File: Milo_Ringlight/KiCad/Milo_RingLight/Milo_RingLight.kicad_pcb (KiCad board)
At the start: 2 copper layers, 16 parts, among them J1 Barrel_Jack_MountingPin, J2 MountingHole, J3 MountingHole, J4 MountingHole, J5 MountingHole, J6 Power Connector

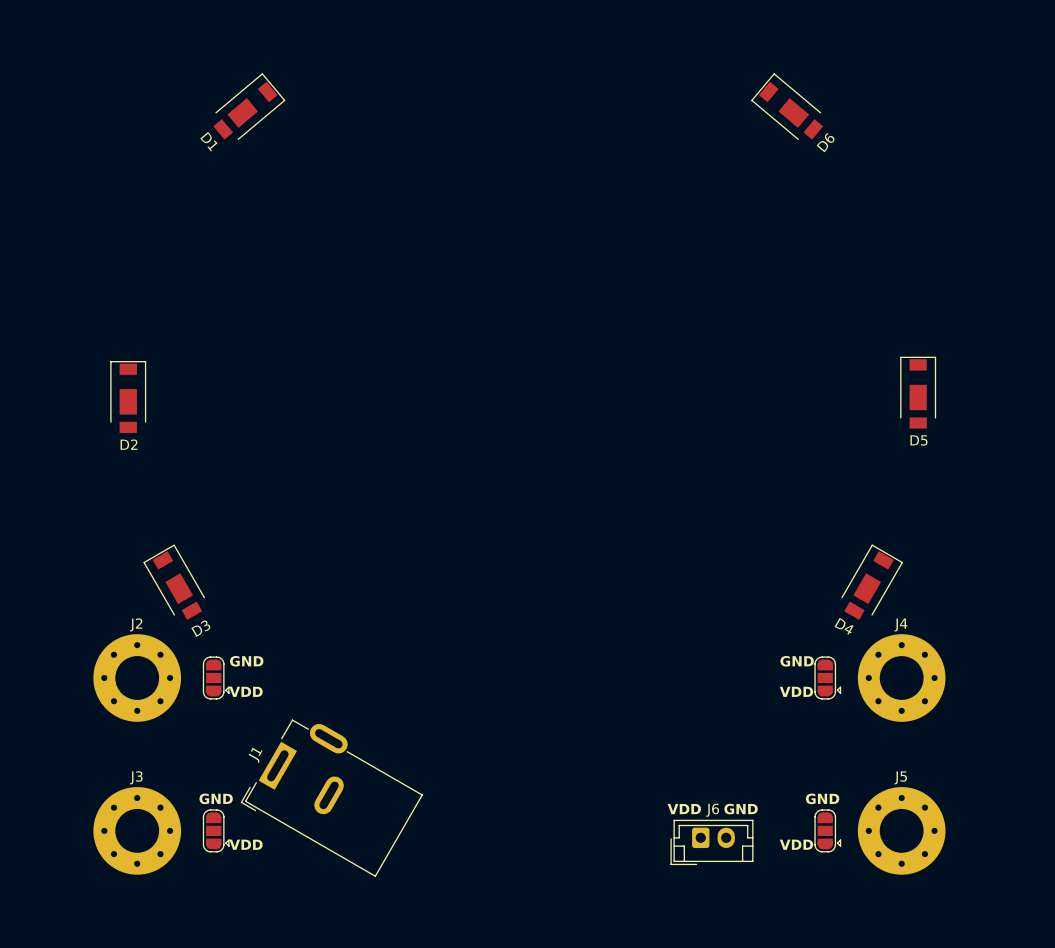
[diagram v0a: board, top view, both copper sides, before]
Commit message: Continued Work.
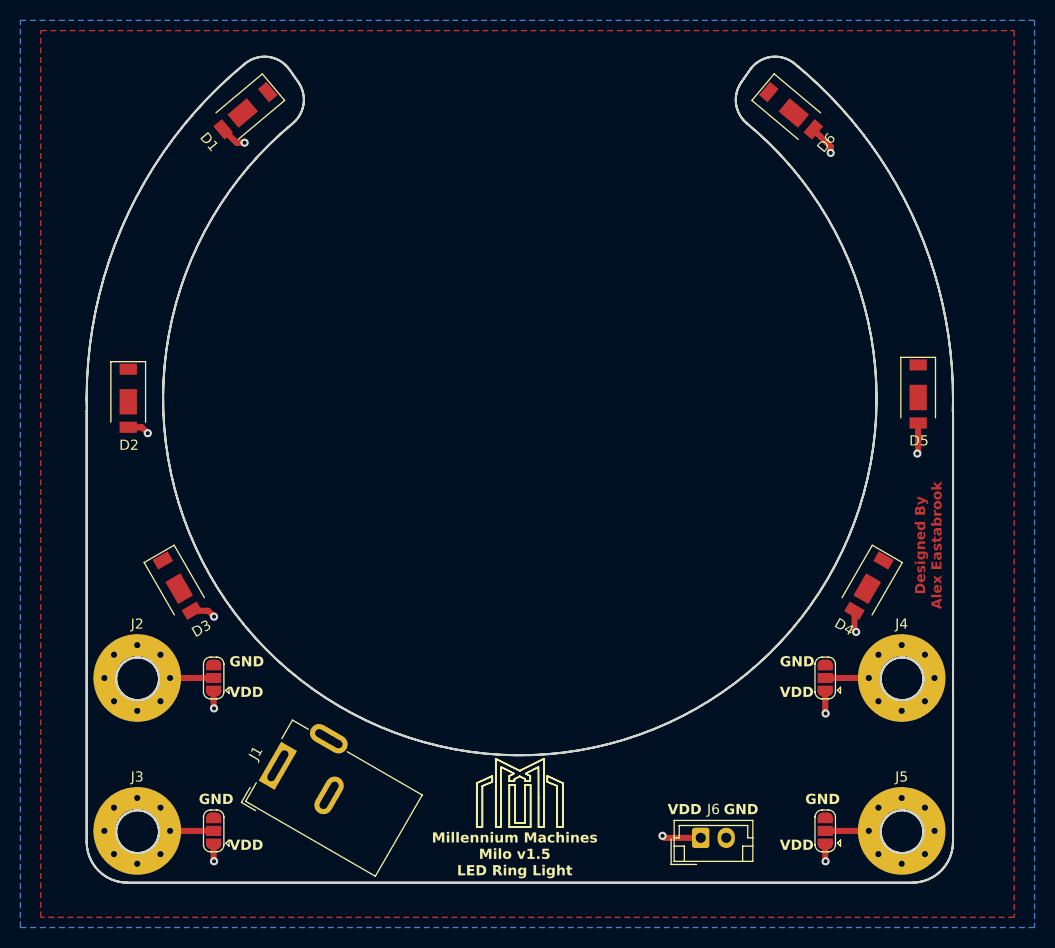
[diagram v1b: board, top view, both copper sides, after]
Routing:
- net VDD: track 0.00 -> 26.5 mm, vias 0 -> 11
- net Net-(J5-Pin_1): track 0.00 -> 4.28 mm
- net Net-(J4-Pin_1): track 0.00 -> 4.28 mm
- net Net-(J3-Pin_1): track 0.00 -> 4.27 mm
- net Net-(J2-Pin_1): track 0.00 -> 4.27 mm
- added copper zone on F.Cu, net GND
- added copper zone on B.Cu, net VDD
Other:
- board outline added: 85 x 81 mm
- board text added: "Designed By Alex Eastabrook"
- board text added: "Millennium Machines Milo v1.5 LED Ring Light"
